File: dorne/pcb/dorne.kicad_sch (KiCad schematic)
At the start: 94 parts, among them J1 MJ-4PP-9, J2 Nice!View, J2 OLED, J3 MJ-4PP-9, J4 OLED, SW1 SW_PUSH, SW10 SW_PUSH, SW11 SW_PUSH, SW12 SW_PUSH, SW13 SW_PUSH, SW14 SW_PUSH, SW15 SW_PUSH, SW16 SW_PUSH, SW17 SW_PUSH, SW18 SW_PUSH, SW19 SW_PUSH, SW2 SW_PUSH, SW20 SW_PUSH, SW21 SW_PUSH, SW22 SW_PUSH, SW23 SW_PUSH, SW24 SW_PUSH, SW25 SW_PUSH, SW26 SW_PUSH, SW27 SW_PUSH, SW28 SW_PUSH, SW29 SW_PUSH, SW3 SW_PUSH, SW30 SW_PUSH, SW31 SW_PUSH, SW32 SW_PUSH, SW33 SW_PUSH, SW34 SW_PUSH, SW35 SW_PUSH, SW36 SW_PUSH, SW37 SW_PUSH, SW38 SW_PUSH, SW39 SW_PUSH, SW4 SW_PUSH, SW40 SW_PUSH, SW41 SW_PUSH, SW42 SW_PUSH, SW5 SW_PUSH, SW6 SW_PUSH, SW7 SW_PUSH, SW8 SW_PUSH, SW9 SW_PUSH, U1 ProMicro, U2 ProMicro, U3 nice_nano

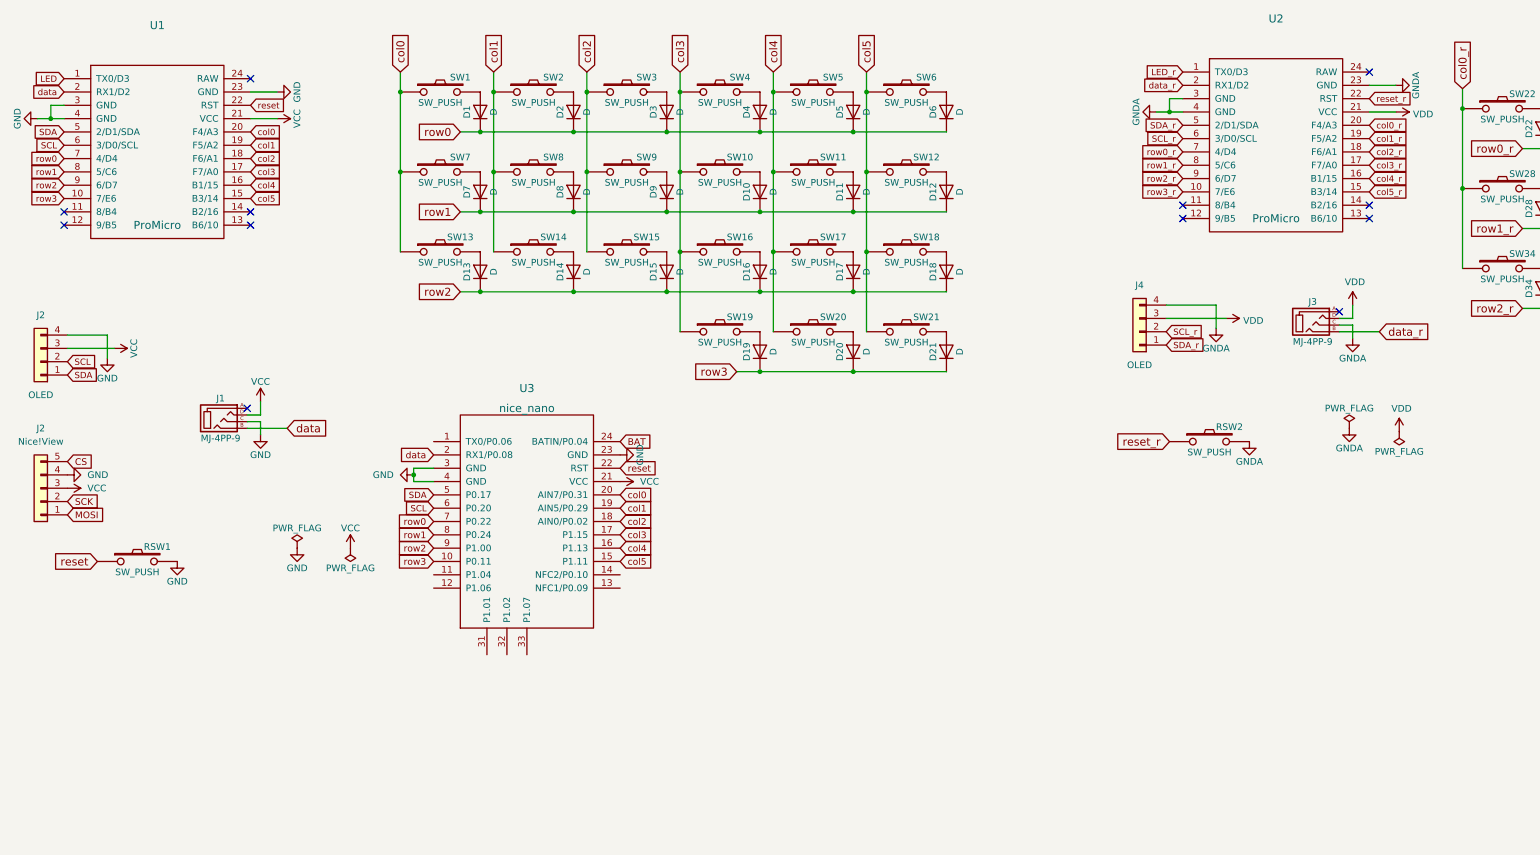
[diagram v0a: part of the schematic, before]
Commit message: Saving state
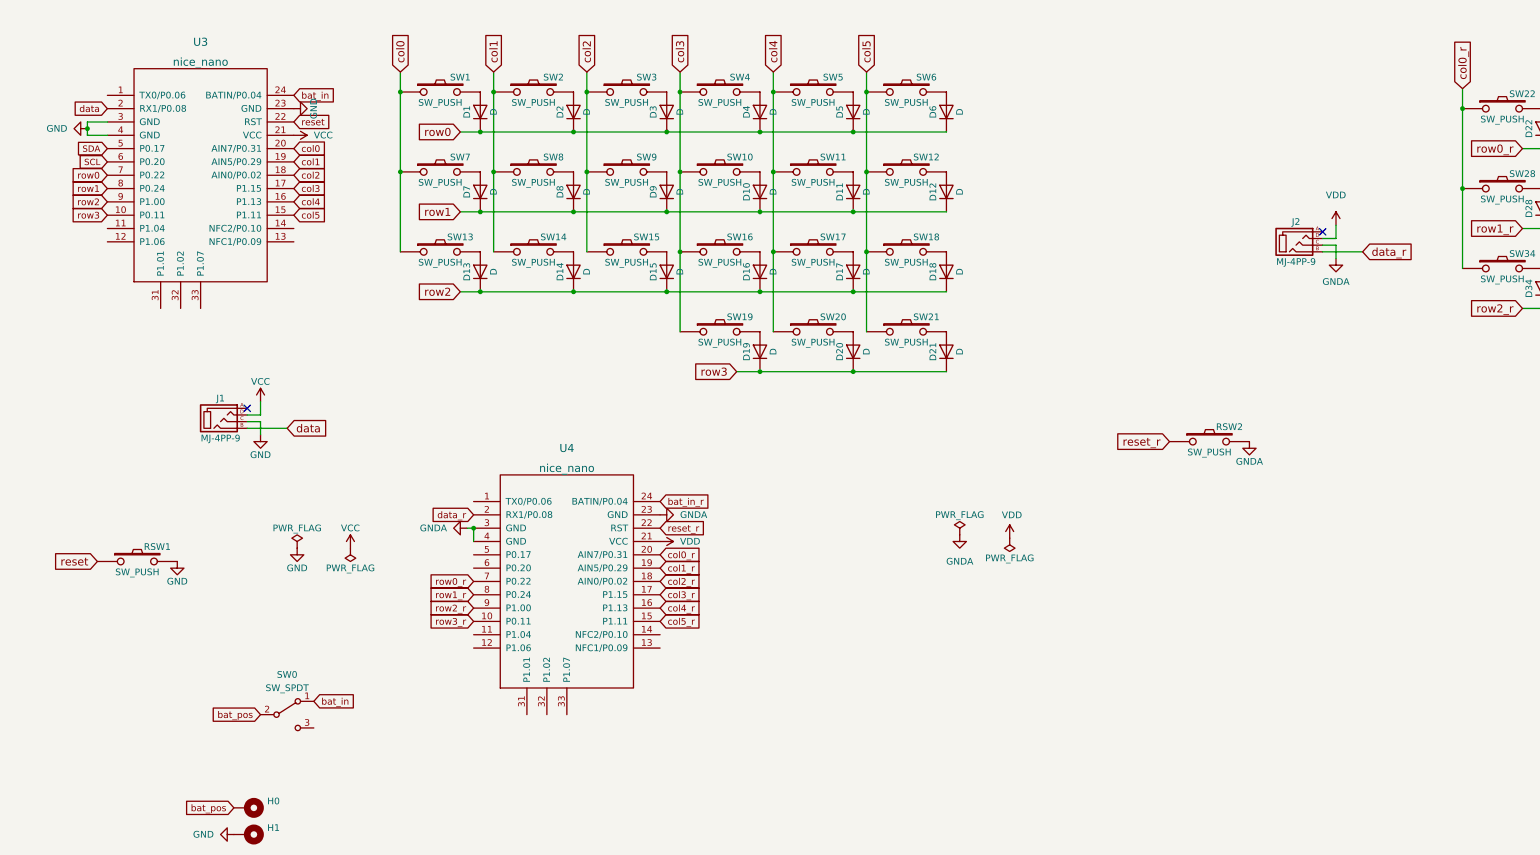
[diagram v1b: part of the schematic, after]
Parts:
- removed J2, J4: OLED, kbd:OLED_1side, symbol Connector_Generic:Conn_01x04
- removed J2: Nice!View, symbol Connector_Generic:Conn_01x05
- removed J3: MJ-4PP-9, kbd:MJ-4PP-9_1side, symbol kbd:MJ-4PP-9
- removed U1, U2: ProMicro, kbd:ProMicro_v3, symbol kbd:ProMicro
- added H0, H1: MountingHole_Pad, Connector_Pin:Pin_D1.0mm_L10.0mm, symbol Mechanical:MountingHole_Pad
- added J2: MJ-4PP-9, kbd:MJ-4PP-9_1side, symbol kbd:MJ-4PP-9
- added SW0: SW_SPDT, lib:ALPS-SSSS811101-0, symbol Switch:SW_SPDT
- added U4: nice_nano, nicenano:nice_nano, symbol nice:nice_nano
- RSW1, RSW2: footprint kbd:ResetSW_1side -> Button_Switch_SMD:SW_Push_SPST_NO_Alps_SKRK
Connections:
- net GND: now also H1.1
- net GNDA: now also J2.C, U4.23 (GND), U4.3 (GND), U4.4 (GND)
- net VDD: now also J2.D, U4.21 (VCC)
- net col0_r: now also U4.20 (AIN7/P0.31)
- net col1_r: now also U4.19 (AIN5/P0.29)
- net col2_r: now also U4.18 (AIN0/P0.02)
- net col3_r: now also U4.17 (P1.15)
- net col4_r: now also U4.16 (P1.13)
- net col5_r: now also U4.15 (P1.11)
- net data_r: now also J2.B, U4.2 (RX1/P0.08)
- net reset_r: now also U4.22 (RST)
- net row0_r: now also U4.7 (P0.22)
- net row1_r: now also U4.8 (P0.24)
- net row2_r: now also U4.9 (P1.00)
- net row3_r: now also U4.10 (P0.11)
- net BAT renamed bat_in
- net bat_in: now also SW0.1 (A)
- new net bat_in_r: U4.24 (BATIN/P0.04)
- new net bat_pos: H0.1, SW0.2 (B)
- no-connect marks 12 -> 2
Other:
- moved on the sheet: U3

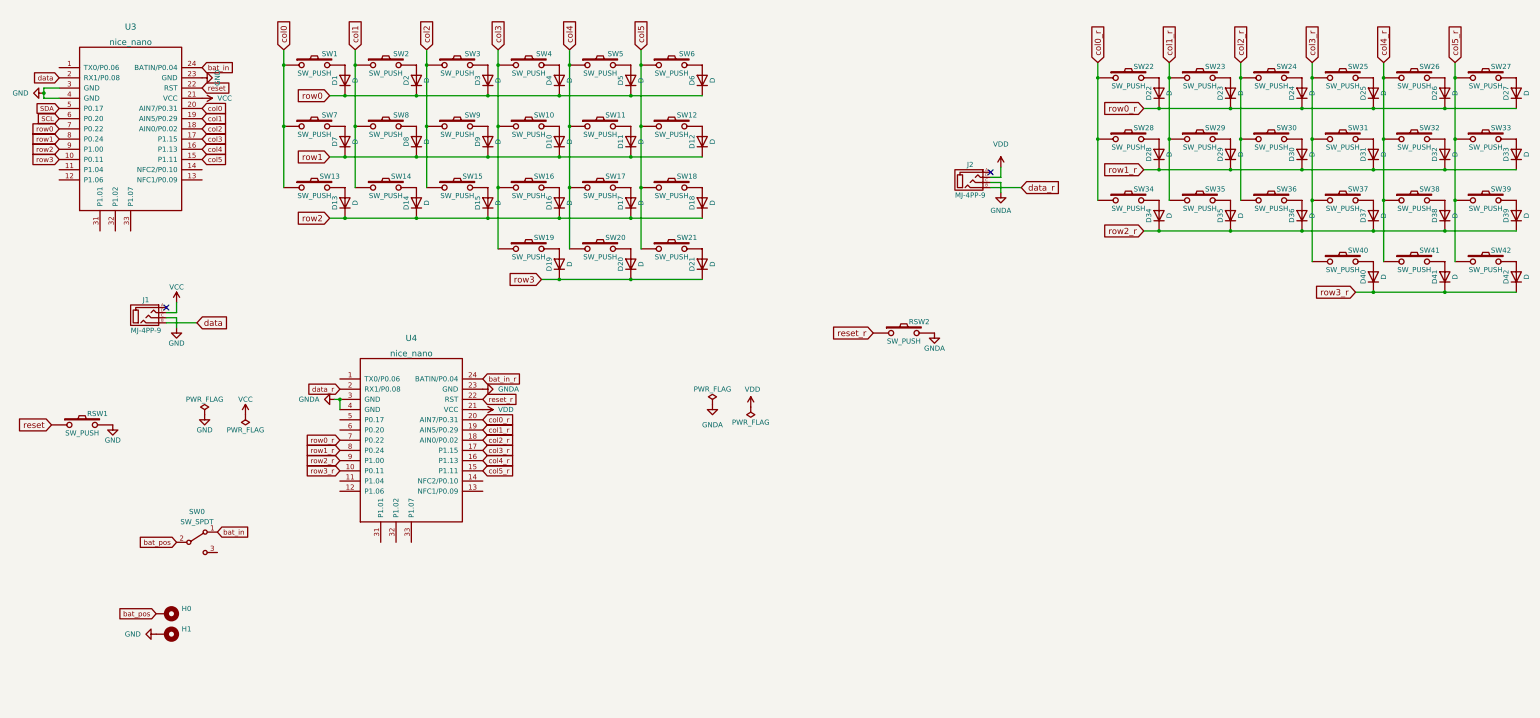
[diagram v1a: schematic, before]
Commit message: Finished everything??
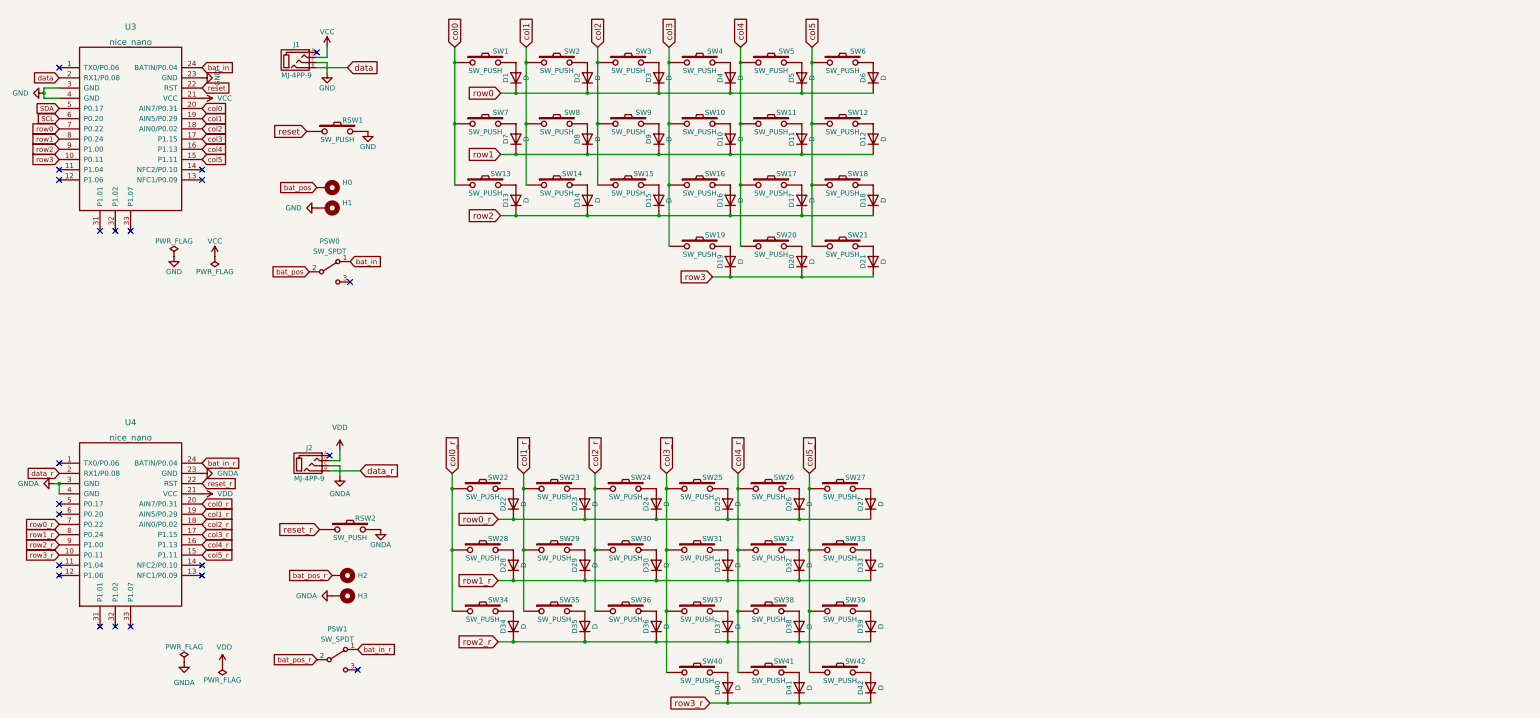
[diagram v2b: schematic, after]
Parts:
- added H2, H3: MountingHole_Pad, Connector_Pin:Pin_D1.0mm_L10.0mm, symbol Mechanical:MountingHole_Pad
- added PSW1: SW_SPDT, lib:ALPS-SSSS811101-0, symbol Switch:SW_SPDT
- renumbered SW0 to PSW0
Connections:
- net GNDA: now also H3.1
- net bat_in_r: now also PSW1.1 (A)
- new net bat_pos_r: H2.1, PSW1.2 (B)
- no-connect marks 2 -> 22
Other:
- moved on the sheet: D1, D10, D11, D12, D13, D14, D15, D16, D17, D18, D19, D2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
